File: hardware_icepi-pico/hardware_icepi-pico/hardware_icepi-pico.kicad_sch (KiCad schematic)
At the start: 3 parts, among them U1 ICE40UP5K-SG48ITR, U2 FT232H, U3 RT6150AGQW

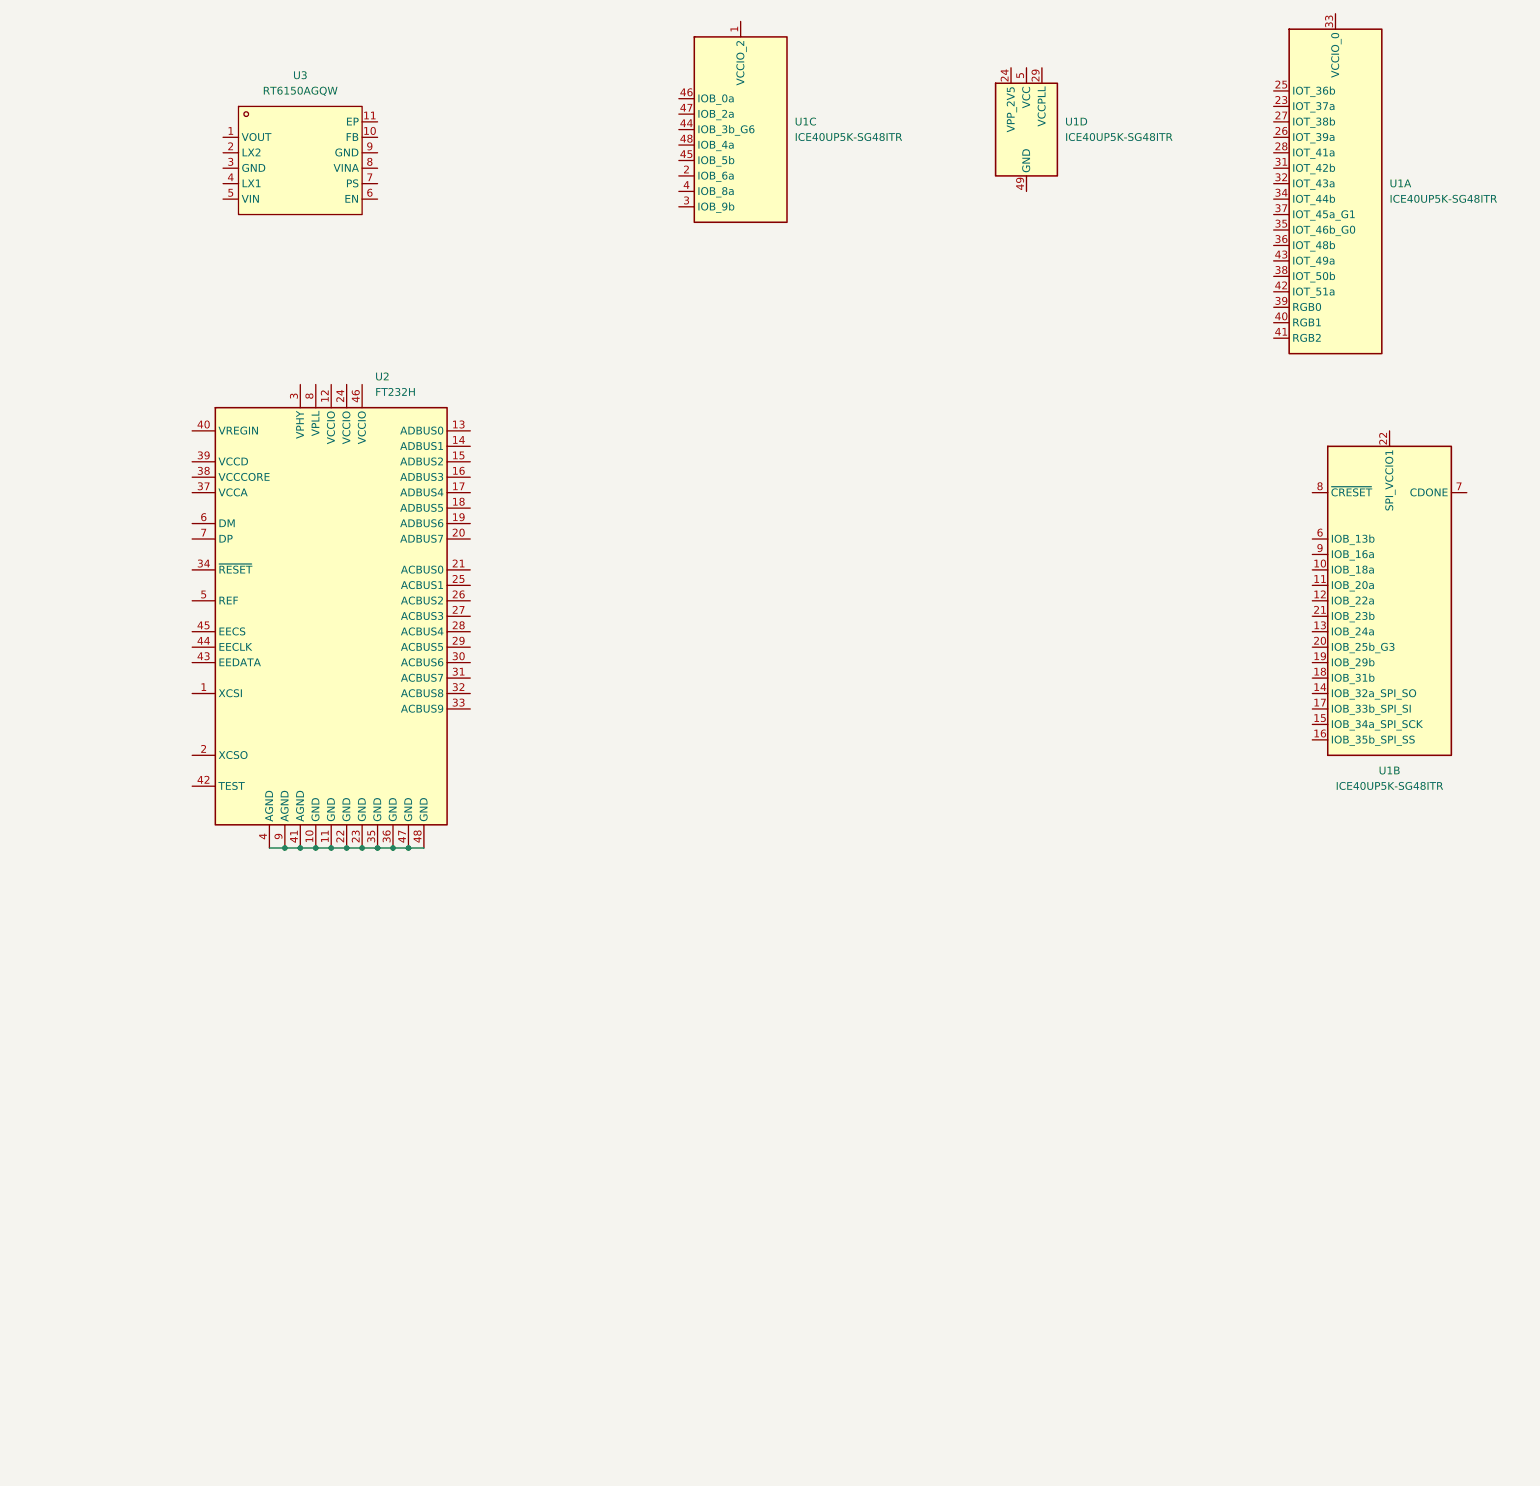
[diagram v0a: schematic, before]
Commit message: sch
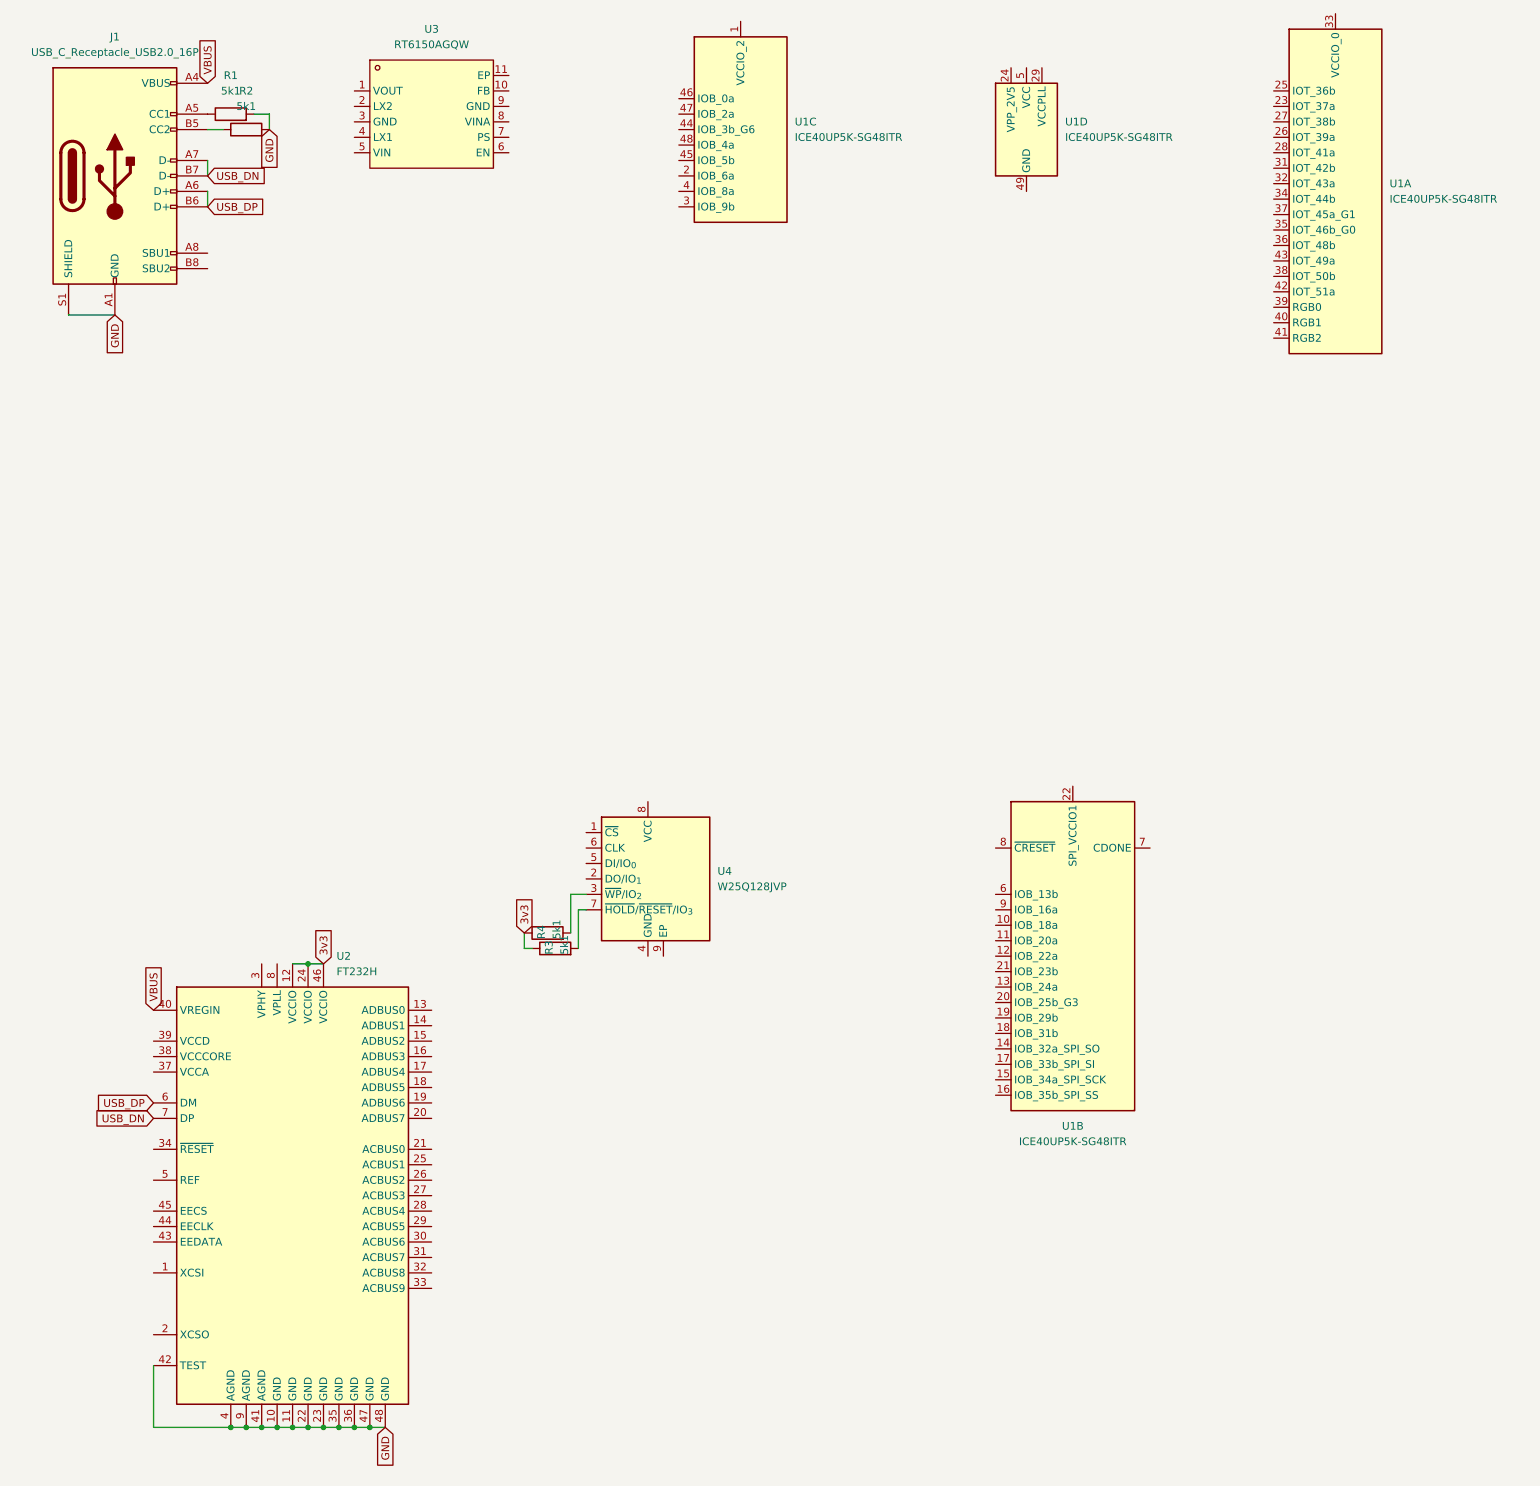
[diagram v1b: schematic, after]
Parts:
- added J1: USB_C_Receptacle_USB2.0_16P, symbol Connector:USB_C_Receptacle_USB2.0_16P
- added R1, R2, R3, R4: 5k1, symbol Device:R
- added U4: W25Q128JVP, Package_SON:WSON-8-1EP_6x5mm_P1.27mm_EP3.4x4.3mm, symbol Memory_Flash:W25Q128JVP
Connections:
- net GND: now reaches U2.10 (GND), U2.11 (GND), U2.22 (GND), U2.23 (GND), U2.35 (GND), U2.36 (GND), U2.4 (AGND), U2.41 (AGND), U2.47 (GND), U2.48 (GND), U2.9 (AGND)
- net GND: now also U2.42 (TEST), J1.A1 (GND), J1.A12 (GND), J1.B1 (GND), J1.B12 (GND), J1.S1 (SHIELD), R1.2, R2.2
- net 3v3: now reaches U2.12 (VCCIO)
- net 3v3: now also U2.24 (VCCIO), U2.46 (VCCIO), R3.1, R4.1
- net VBUS: now reaches U2.40 (VREGIN)
- net VBUS: now also J1.A4 (VBUS), J1.A9 (VBUS), J1.B4 (VBUS), J1.B9 (VBUS)
- net USB_DP: now reaches U2.6 (DM)
- net USB_DP: now also J1.A6 (D+), J1.B6 (D+)
- net USB_DN: now reaches U2.7 (DP)
- net USB_DN: now also J1.A7 (D-), J1.B7 (D-)
- new net: J1.B5 (CC2), R2.1
- new net: R4.2, U4.3 (~{WP}/IO_{2})
- new net: R3.2, U4.7 (~{HOLD}/~{RESET}/IO_{3})
- new net: J1.A5 (CC1), R1.1
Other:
- moved on the sheet: U1B, U2, U3
